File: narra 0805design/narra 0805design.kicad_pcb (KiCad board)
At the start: 2 copper layers, 61 x 11.7 mm, 18 parts, among them J1 Rows, J2 Columns

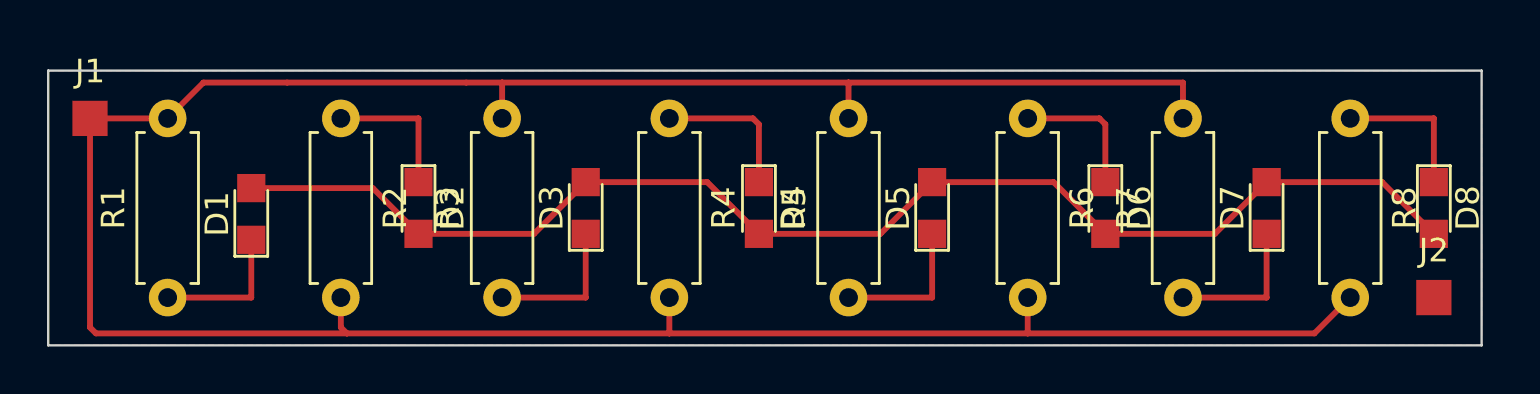
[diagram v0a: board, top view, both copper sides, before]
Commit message: finalise matrix column design prior to meshing design
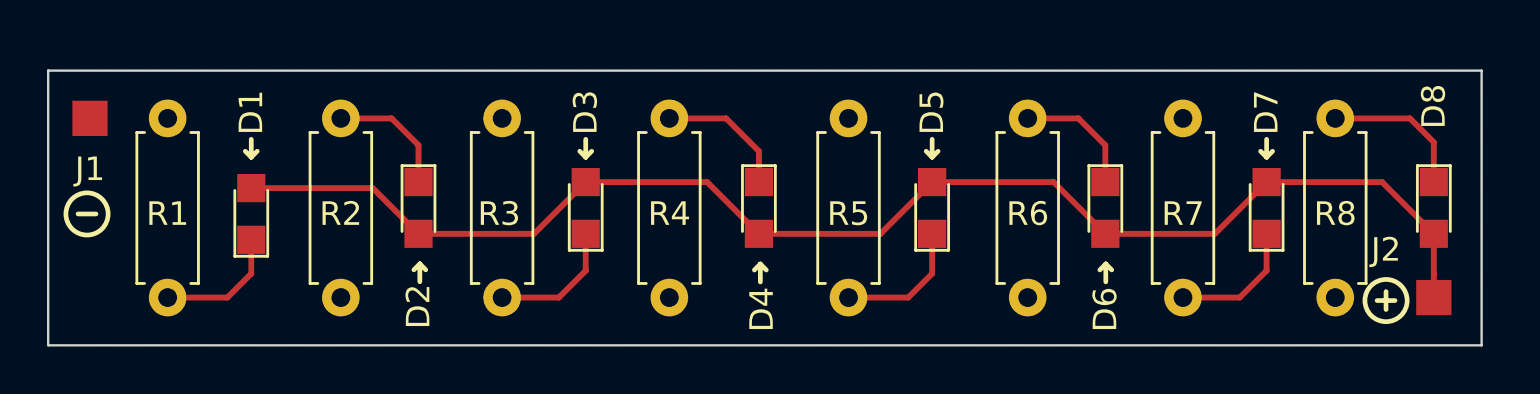
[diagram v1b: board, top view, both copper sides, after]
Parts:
- moved R8 0.63 mm to (204.1, 84.8)
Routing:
- net GNDREF: track 119.6 -> 0.00 mm
- net /C: track 56.6 -> 59.3 mm
- net Net-(D7-Pad1): track 6.27 -> 5.60 mm
- net Net-(D4-Pad1): track 6.37 -> 5.70 mm
- net Net-(D3-Pad1): track 6.27 -> 5.60 mm
- net Net-(D2-Pad1): track 6.01 -> 5.34 mm
- net Net-(D5-Pad1): track 6.27 -> 5.67 mm
- net Net-(D1-Pad1): track 6.01 -> 5.42 mm
- net Net-(D6-Pad1): track 5.86 -> 5.34 mm
